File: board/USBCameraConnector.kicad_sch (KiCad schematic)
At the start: 6 parts, among them J1 USB4105-GF-A, J7 Conn_01x04_Pin

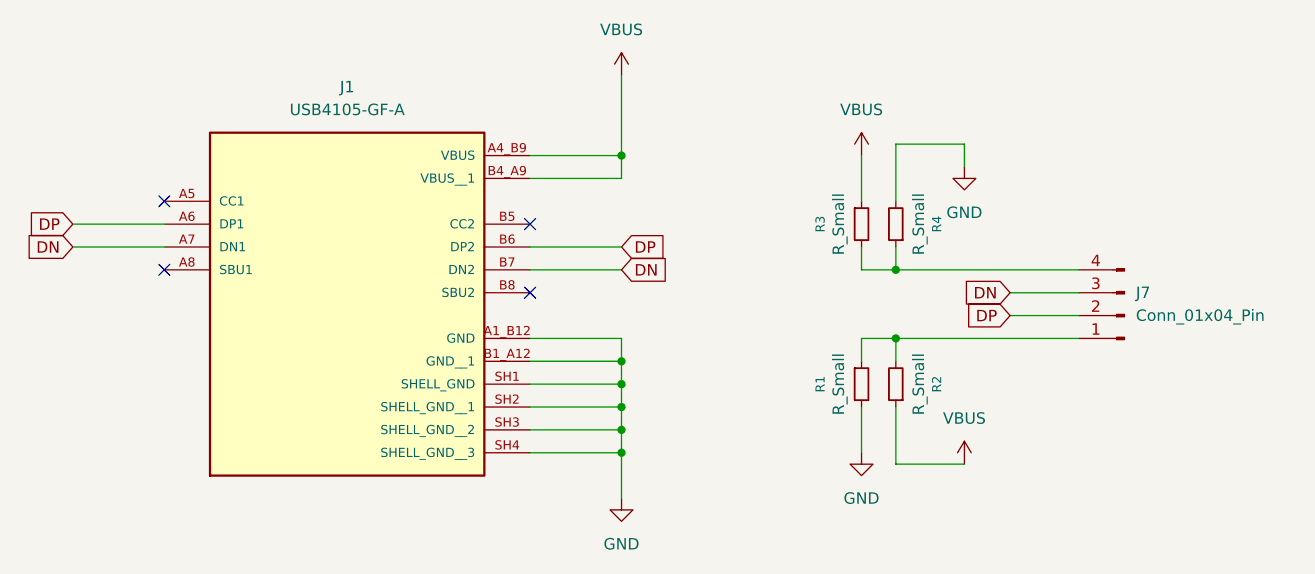
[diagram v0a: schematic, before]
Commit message: Done
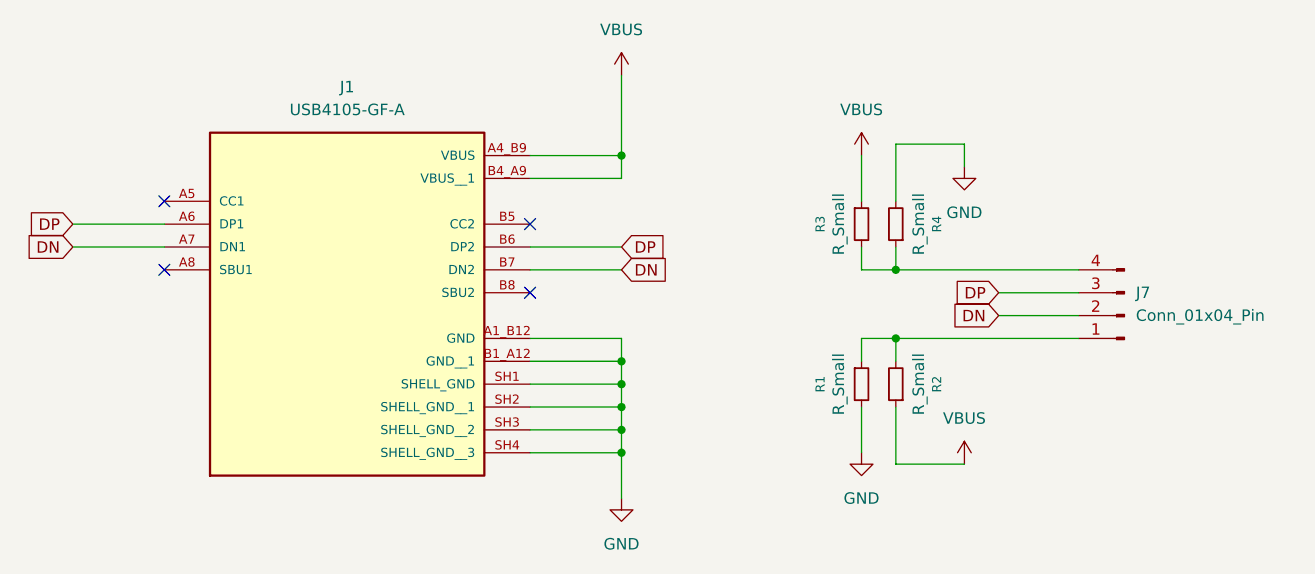
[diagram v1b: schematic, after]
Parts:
- J7: footprint Connector_PinHeader_2.54mm:PinHeader_1x04_P2.54mm_Vertical -> Connector_PinHeader_2.00mm:PinHeader_1x04_P2.00mm_Vertical
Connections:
- net DN: now also J7.2 (Pin_2); no longer J7.3 (Pin_3)
- net DP: now also J7.3 (Pin_3); no longer J7.2 (Pin_2)
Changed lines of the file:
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@@
+	(wire
+		(pts
+			(xy 199.39 83.82) (xy 208.28 83.82)
+		)
+		(stroke
+			(width 0)
+			(type default)
+		)
+	)
+	(wire
+		(pts
+			(xy 199.39 81.28) (xy 208.28 81.28)
+		)
+		(stroke
+			(width 0)
+			(type default)
+		)
+	)
 	(wire
 		(pts
@@
 		(pts
 			(xy 147.32 66.04) (xy 157.48 66.04)
-		)
-		(stroke
-			(width 0)
-			(type default)
-		)
-	)
-	(wire
-		(pts
-			(xy 200.66 81.28) (xy 208.28 81.28)
-		)
-		(stroke
-			(width 0)
-			(type default)
-		)
-	)
-	(wire
-		(pts
-			(xy 200.66 83.82) (xy 208.28 83.82)
 		)
 		(stroke
@@
 	(global_label "DN"
 		(shape input)
-		(at 200.66 81.28 180)
+		(at 199.39 83.82 180)
 		(fields_autoplaced yes)
 		(effects
@@
 		)
 		(property "Intersheetrefs" "${INTERSHEET_REFS}"
-			(at 195.0743 81.28 0)
+			(at 193.8043 83.82 0)
 			(effects
 				(font
@@
 	(global_label "DP"
 		(shape input)
-		(at 200.66 83.82 180)
+		(at 199.39 81.28 180)
 		(fields_autoplaced yes)
 		(effects
@@
 		)
 		(property "Intersheetrefs" "${INTERSHEET_REFS}"
-			(at 195.1348 83.82 0)
+			(at 193.8648 81.28 0)
 			(effects
 				(font
@@
 			)
 		)
-		(property "Footprint" "Connector_PinHeader_2.54mm:PinHeader_1x04_P2.54mm_Vertical"
+		(property "Footprint" "Connector_PinHeader_2.00mm:PinHeader_1x04_P2.00mm_Vertical"
 			(at 213.36 83.82 0)
 			(effects
